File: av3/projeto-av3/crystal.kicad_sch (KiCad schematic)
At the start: 2 parts, among them SW17 SW_Push

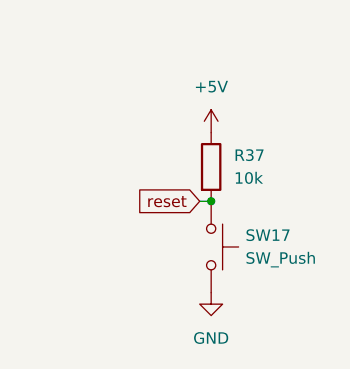
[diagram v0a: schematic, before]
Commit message: Esquemático finalizado, faltando somente o PCB.
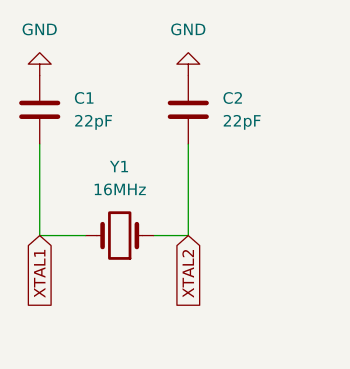
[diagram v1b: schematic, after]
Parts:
- removed R37: 10k, Resistor_SMD:R_1206_3216Metric_Pad1.30x1.75mm_HandSolder, symbol Device:R
- removed SW17: SW_Push, Button_Switch_THT:SW_PUSH_6mm_H4.3mm, symbol Switch:SW_Push
- added C1, C2: 22pF, Capacitor_SMD:C_1206_3216Metric, symbol Device:C
- added Y1: 16MHz, Crystal:Crystal_SMD_HC49-SD, symbol Device:Crystal
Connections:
- net GND: now also C1.2, C2.2
- new net XTAL1: C1.1, Y1.2
- new net XTAL2: C2.1, Y1.1
